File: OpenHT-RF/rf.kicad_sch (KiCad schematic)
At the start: 37 parts, among them J501 EMPCB.CSMAFSTJ.A, J502 Conn_01x02, J503 Conn_01x02, SW501 RFSW8008, U501 AT86RF215, X501 ECS-TXO-20CSMV

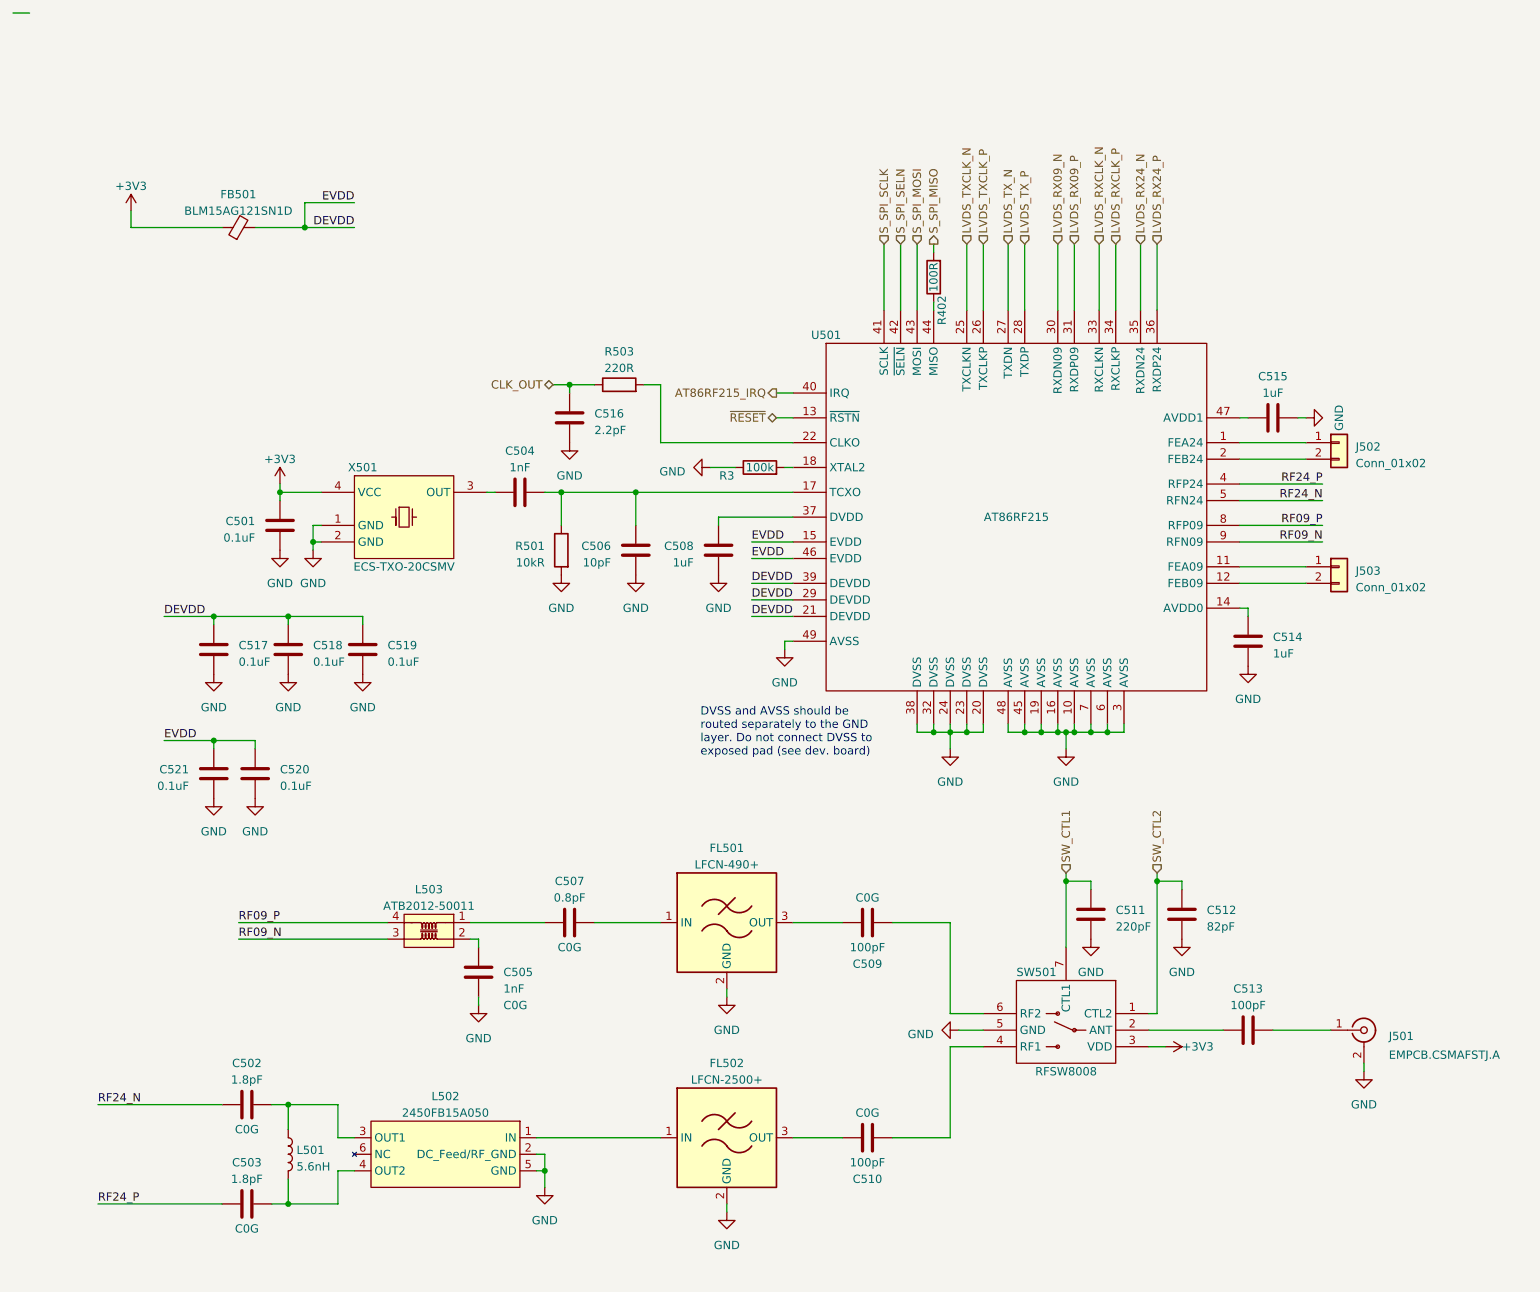
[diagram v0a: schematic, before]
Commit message: Various schematic updates
Edited IO names, updated load switch symbol, swapped RF switch inputs
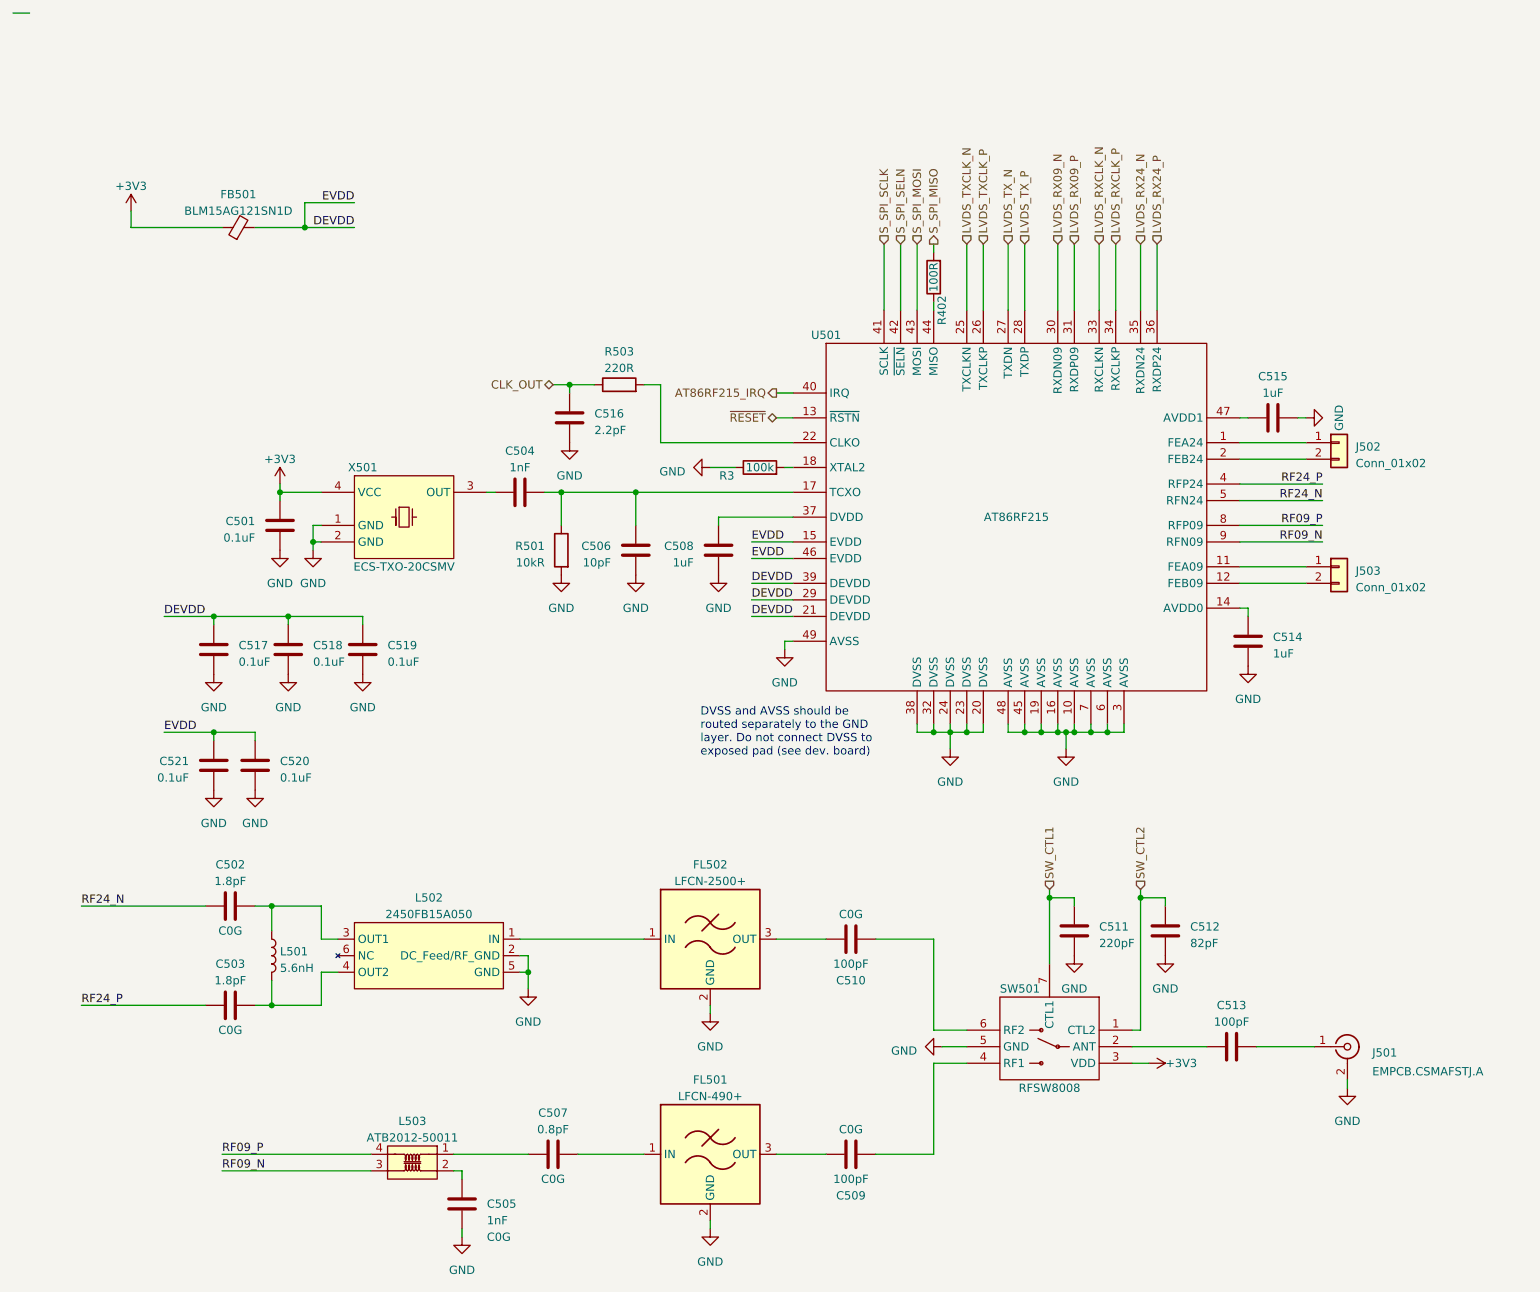
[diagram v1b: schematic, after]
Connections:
- net at C509.2: now also SW501.4 (RF1); no longer SW501.6 (RF2)
- net at C510.2: now also SW501.6 (RF2); no longer SW501.4 (RF1)
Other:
- moved on the sheet: C502, C503, C505, C507, C509, C510, C511, C512, C513, C520, C521, FL501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
